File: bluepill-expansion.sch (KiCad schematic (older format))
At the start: 1 part, among them U1 BluePill_STM32F103C

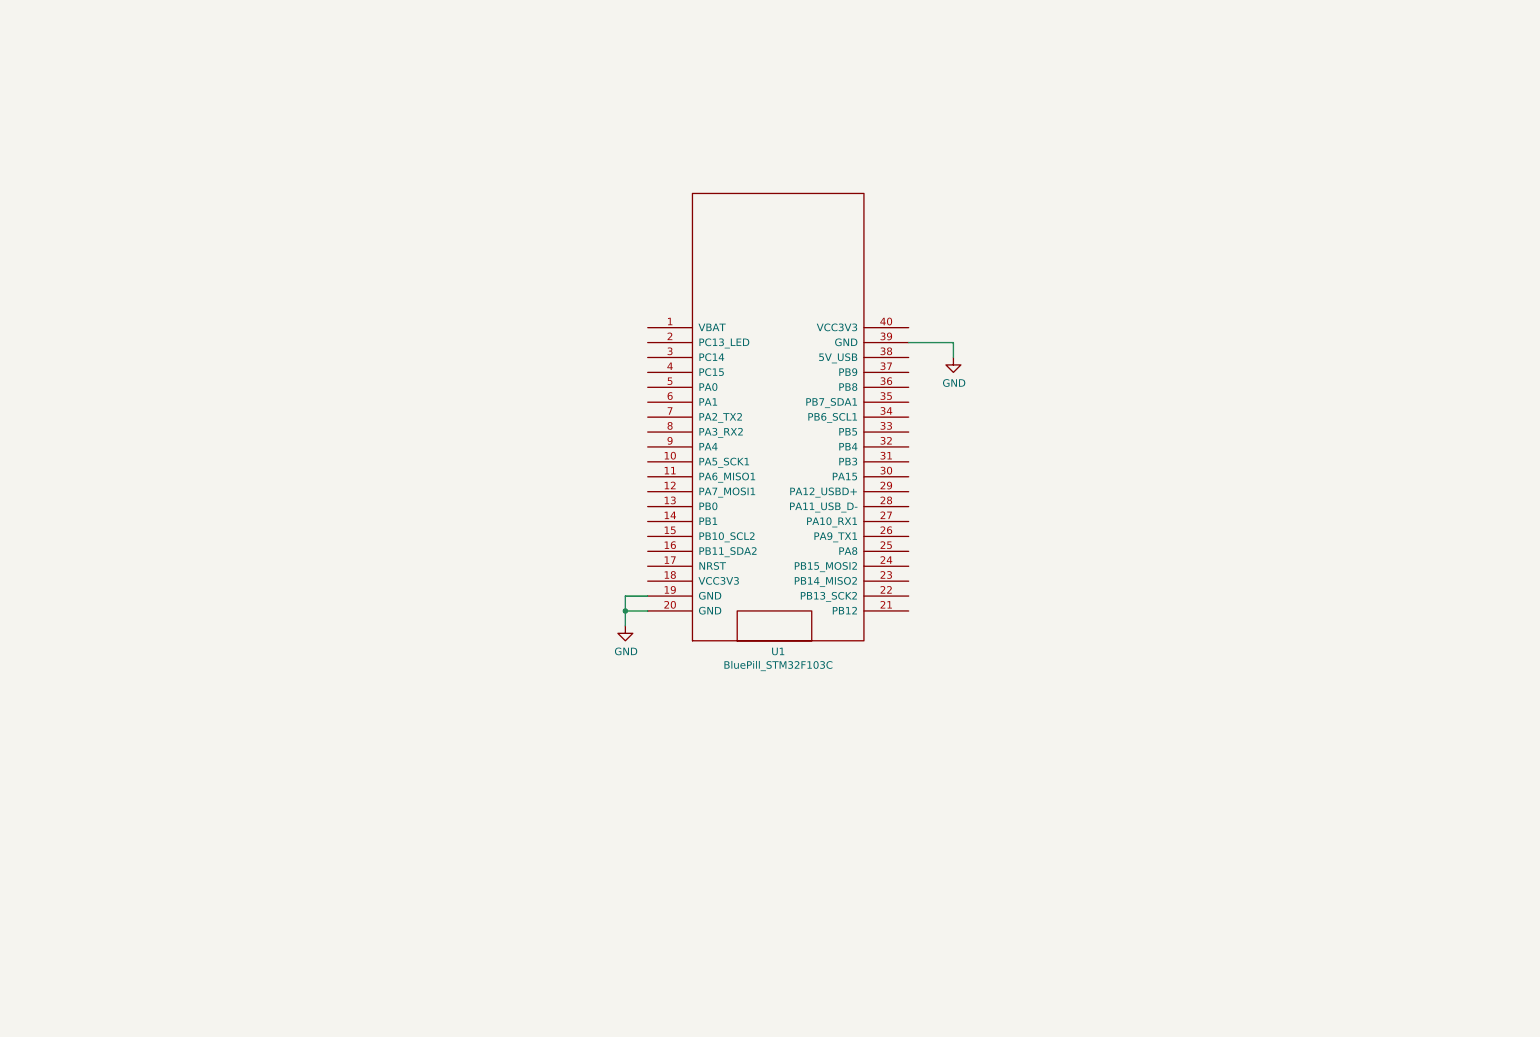
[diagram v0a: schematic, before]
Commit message: project update
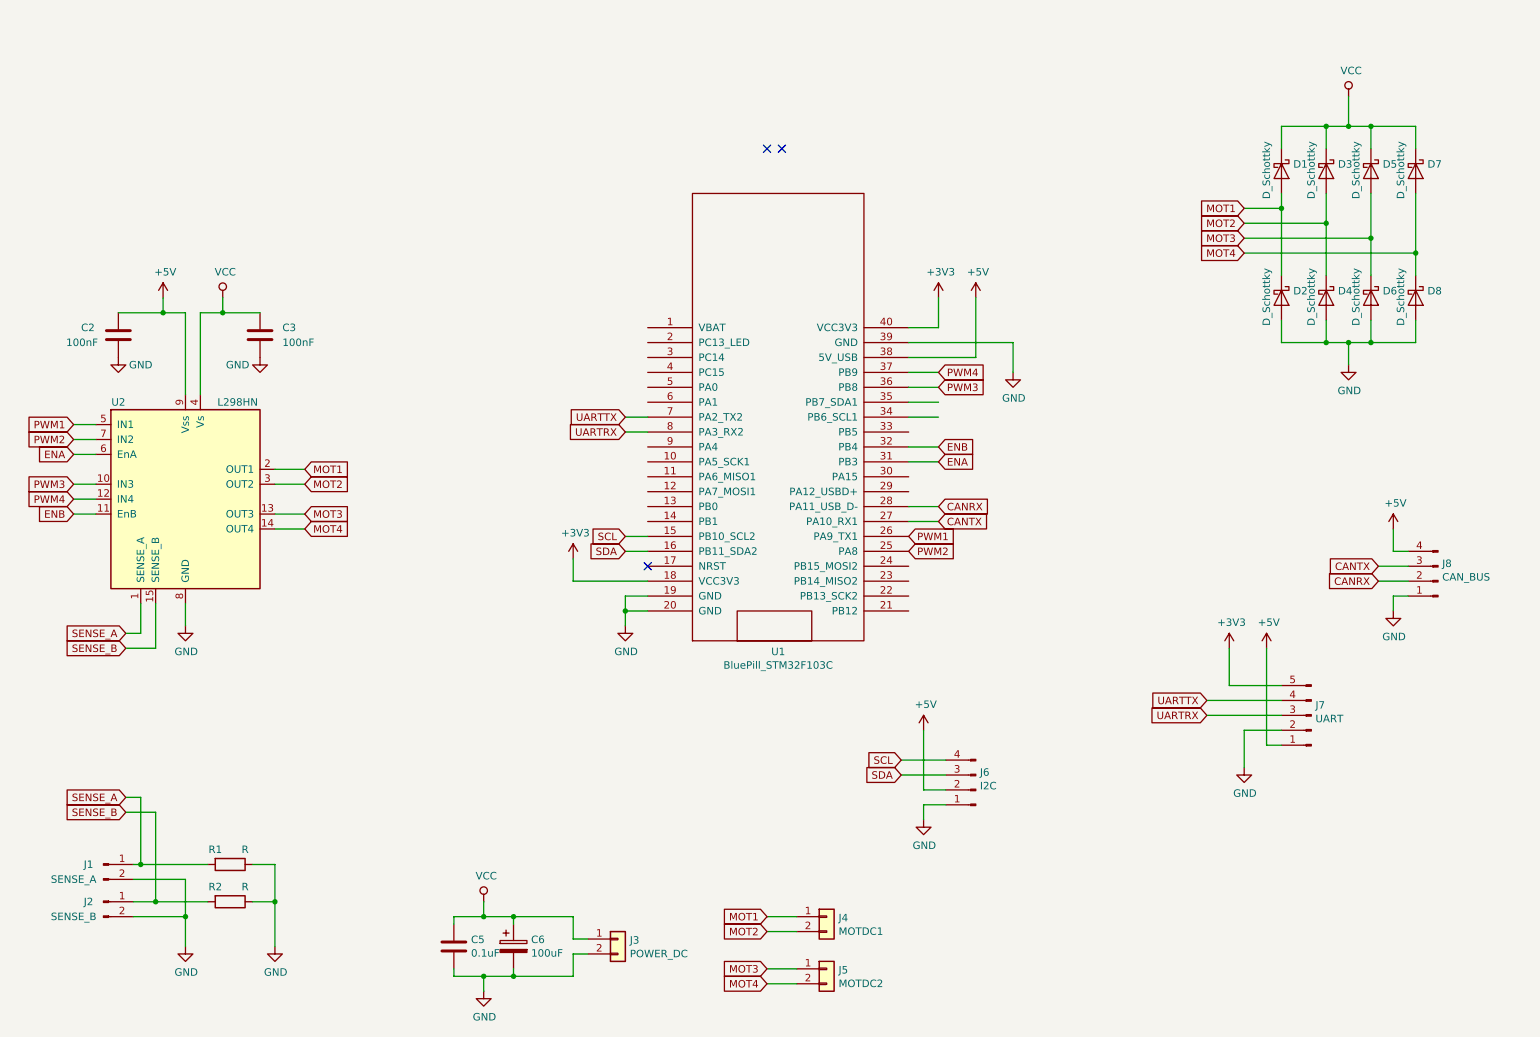
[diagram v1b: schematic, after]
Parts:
- added C2, C3: 100nF, symbol Device:C
- added C5: 0.1uF, Capacitor_THT:C_Disc_D7.5mm_W2.5mm_P5.00mm, symbol Device:C
- added C6: 100uF, Capacitor_THT:CP_Radial_D5.0mm_P2.50mm, symbol Device:CP
- added D1, D2, D3, D4, D5, D6, D7, D8: D_Schottky, symbol Device:D_Schottky
- added J1: SENSE_A, Connector_PinHeader_2.54mm:PinHeader_1x02_P2.54mm_Vertical, symbol Connector:Conn_01x02_Male
- added J2: SENSE_B, Connector_PinHeader_2.54mm:PinHeader_1x02_P2.54mm_Vertical, symbol Connector:Conn_01x02_Male
- added J3: POWER_DC, TerminalBlock:TerminalBlock_bornier-2_P5.08mm, symbol Connector_Generic:Conn_01x02
- added J4: MOTDC1, TerminalBlock:TerminalBlock_bornier-2_P5.08mm, symbol Connector_Generic:Conn_01x02
- added J5: MOTDC2, TerminalBlock:TerminalBlock_bornier-2_P5.08mm, symbol Connector_Generic:Conn_01x02
- added J6: I2C, Connector_PinHeader_2.54mm:PinHeader_1x04_P2.54mm_Vertical, symbol Connector:Conn_01x04_Male
- added J7: UART, Connector_PinHeader_2.54mm:PinHeader_1x05_P2.54mm_Vertical, symbol Connector:Conn_01x05_Male
- added J8: CAN_BUS, Connector_PinHeader_2.54mm:PinHeader_1x04_P2.54mm_Vertical, symbol Connector:Conn_01x04_Male
- added R1, R2: R, symbol Device:R
- added U2: L298HN, Package_TO_SOT_THT:TO-220-15_P2.54x2.54mm_StaggerOdd_Lead4.58mm_Vertical, symbol Driver_Motor:L298HN
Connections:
- net GND: now also C2.2, C3.2, C5.2, C6.2, D2.2 (A), D4.2 (A), D6.2 (A), D8.2 (A), J1.2 (Pin_2), J2.2 (Pin_2), J3.2 (Pin_2), J6.1 (Pin_1), J7.2 (Pin_2), J8.1 (Pin_1), R1.1, R2.1, U2.8 (GND)
- net SCL: now reaches U1.15 (PB10_SCL2)
- net SCL: now also J6.4 (Pin_4)
- net SDA: now reaches U1.16 (PB11_SDA2)
- net SDA: now also J6.3 (Pin_3)
- net +3V3: now reaches U1.18 (VCC3V3)
- net +3V3: now also U1.40 (VCC3V3), J7.5 (Pin_5)
- net PWM2: now reaches U1.25 (PA8)
- net PWM2: now also U2.7 (IN2)
- net PWM1: now reaches U1.26 (PA9_TX1)
- net PWM1: now also U2.5 (IN1)
- net CANTX: now reaches U1.27 (PA10_RX1)
- net CANTX: now also J8.3 (Pin_3)
- net CANRX: now reaches U1.28 (PA11_USB_D-)
- net CANRX: now also J8.2 (Pin_2)
- net ENA: now reaches U1.31 (PB3)
- net ENA: now also U2.6 (EnA)
- net ENB: now reaches U1.32 (PB4)
- net ENB: now also U2.11 (EnB)
- net PWM3: now reaches U1.36 (PB8)
- net PWM3: now also U2.10 (IN3)
- net PWM4: now reaches U1.37 (PB9)
- net PWM4: now also U2.12 (IN4)
- net +5V: now reaches U1.38 (5V_USB)
- net +5V: now also C2.1, J6.2 (Pin_2), J7.1 (Pin_1), J8.4 (Pin_4), U2.9 (Vss)
- net UARTTX: now reaches U1.7 (PA2_TX2)
- net UARTTX: now also J7.4 (Pin_4)
- net UARTRX: now reaches U1.8 (PA3_RX2)
- net UARTRX: now also J7.3 (Pin_3)
- new net MOT1: D1.2 (A), D2.1 (K), J4.1 (Pin_1), U2.2 (OUT1)
- new net MOT2: D3.2 (A), D4.1 (K), J4.2 (Pin_2), U2.3 (OUT2)
- new net MOT3: D5.2 (A), D6.1 (K), J5.1 (Pin_1), U2.13 (OUT3)
- new net MOT4: D7.2 (A), D8.1 (K), J5.2 (Pin_2), U2.14 (OUT4)
- new net SENSE_A: J1.1 (Pin_1), R1.2, U2.1 (SENSE_A)
- new net SENSE_B: J2.1 (Pin_1), R2.2, U2.15 (SENSE_B)
- new net VCC: C3.1, C5.1, C6.1, D1.1 (K), D3.1 (K), D5.1 (K), D7.1 (K), J3.1 (Pin_1), U2.4 (Vs)
- no-connect marks 0 -> 3

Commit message: updated schematic
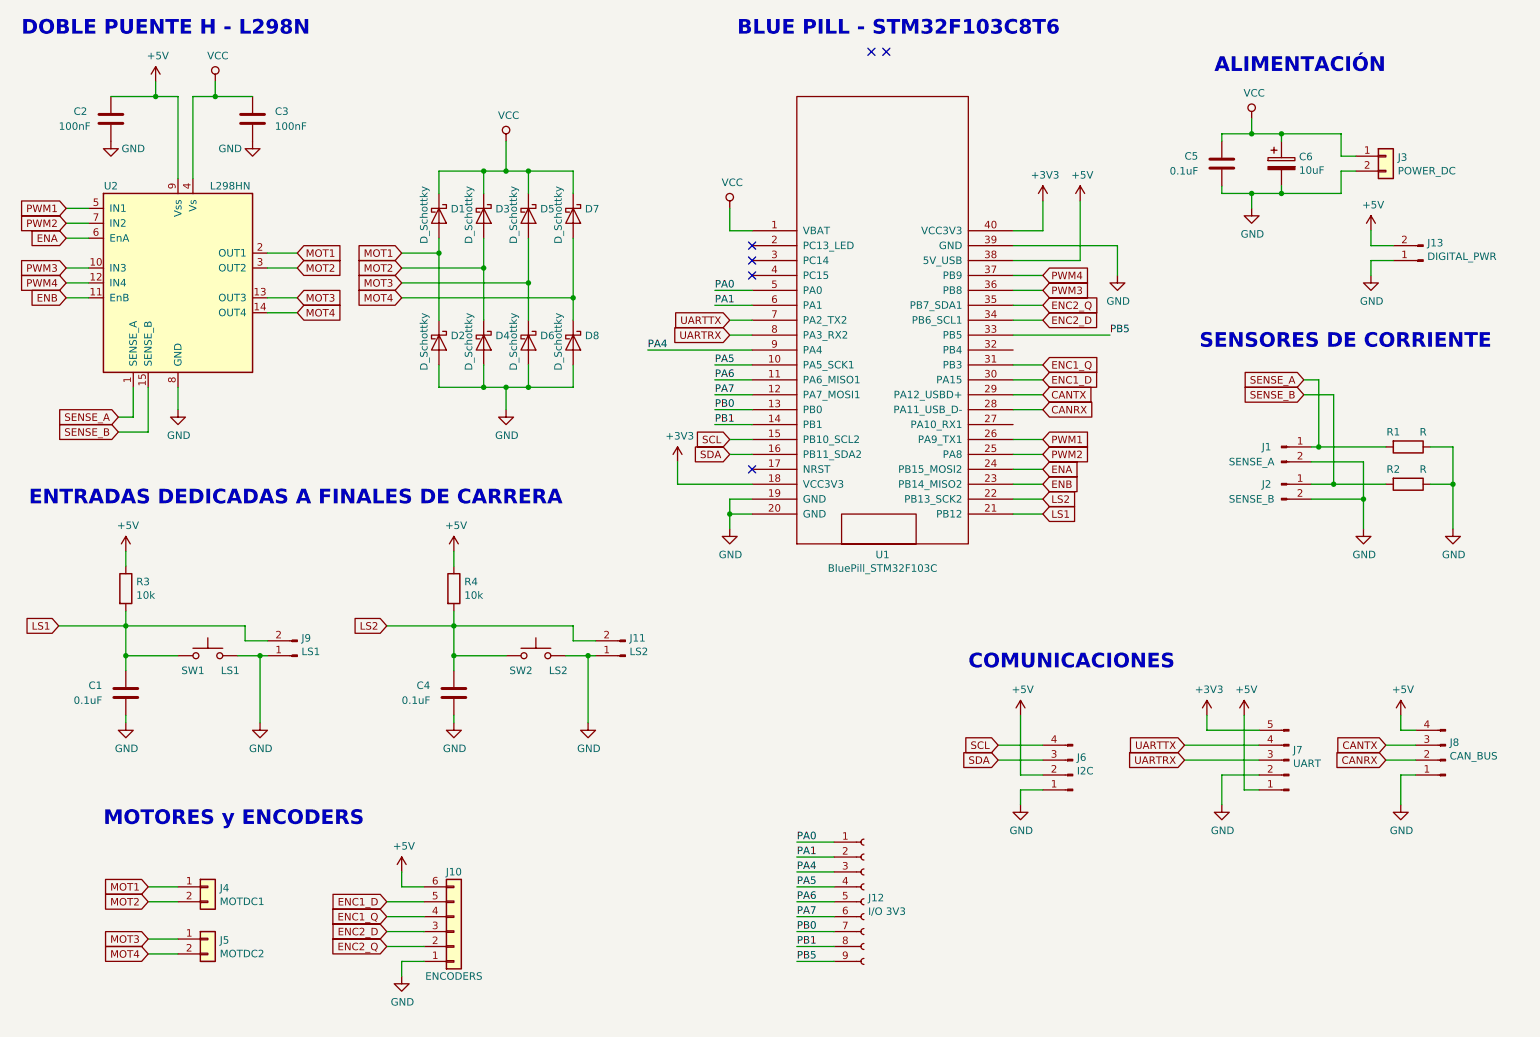
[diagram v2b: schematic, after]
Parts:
- added C1: 0.1uF, Capacitor_THT:C_Disc_D7.5mm_W2.5mm_P5.00mm, symbol Device:C
- added C4: 0.1uF, Capacitor_THT:C_Disc_D7.0mm_W2.5mm_P5.00mm, symbol Device:C
- added J10: ENCODERS, TerminalBlock:TerminalBlock_bornier-6_P5.08mm, symbol Connector_Generic:Conn_01x06
- added J11: LS2, Connector_PinHeader_2.54mm:PinHeader_1x02_P2.54mm_Vertical, symbol Connector:Conn_01x02_Male
- added J12: I/O 3V3, Connector_PinSocket_2.54mm:PinSocket_1x09_P2.54mm_Vertical, symbol Connector:Conn_01x09_Female
- added J13: DIGITAL_PWR, Connector_PinHeader_2.54mm:PinHeader_1x02_P2.54mm_Vertical, symbol Connector:Conn_01x02_Male
- added J9: LS1, Connector_PinHeader_2.54mm:PinHeader_1x02_P2.54mm_Vertical, symbol Connector:Conn_01x02_Male
- added R3, R4: 10k, Resistor_THT:R_Axial_DIN0207_L6.3mm_D2.5mm_P10.16mm_Horizontal, symbol Device:R
- added SW1: LS1, Button_Switch_THT:SW_PUSH_6mm_H8.5mm, symbol Switch:SW_Push
- added SW2: LS2, Button_Switch_THT:SW_PUSH_6mm_H8.5mm, symbol Switch:SW_Push
- C2, C3: footprint (none) -> Capacitor_THT:C_Disc_D7.5mm_W2.5mm_P5.00mm
- C6: value 100uF -> 10uF
- D1, D2, D3, D4, D5, D6, D7, D8: footprint (none) -> Diode_THT:D_DO-41_SOD81_P12.70mm_Horizontal
- R1, R2: footprint (none) -> Resistor_THT:R_Box_L26.0mm_W5.0mm_P20.00mm
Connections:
- net +5V: now also J10.6 (Pin_6), J13.2 (Pin_2), R3.1, R4.1
- net CANTX: now also U1.29 (PA12_USBD+); no longer U1.27 (PA10_RX1)
- net ENA: now also U1.24 (PB15_MOSI2); no longer U1.31 (PB3)
- net ENB: now also U1.23 (PB14_MISO2); no longer U1.32 (PB4)
- net GND: now also C1.2, C4.2, J10.1 (Pin_1), J11.1 (Pin_1), J13.1 (Pin_1), J9.1 (Pin_1), SW1.2, SW2.2
- net VCC: now also U1.1 (VBAT)
- net PA5: now reaches U1.10 (PA5_SCK1)
- net PA5: now also J12.4 (Pin_4)
- net PA6: now reaches U1.11 (PA6_MISO1)
- net PA6: now also J12.5 (Pin_5)
- net PA7: now reaches U1.12 (PA7_MOSI1)
- net PA7: now also J12.6 (Pin_6)
- net PB0: now reaches U1.13 (PB0)
- net PB0: now also J12.7 (Pin_7)
- net PB1: now reaches U1.14 (PB1)
- net PB1: now also J12.8 (Pin_8)
- net LS1: now reaches U1.21 (PB12)
- net LS1: now also C1.1, J9.2 (Pin_2), R3.2, SW1.1
- net LS2: now reaches U1.22 (PB13_SCK2)
- net LS2: now also C4.1, J11.2 (Pin_2), R4.2, SW2.1
- net ENC1_D: now reaches U1.30 (PA15)
- net ENC1_D: now also J10.5 (Pin_5)
- net PB5: now reaches U1.33 (PB5)
- net PB5: now also J12.9 (Pin_9)
- net ENC2_D: now reaches U1.34 (PB6_SCL1)
- net ENC2_D: now also J10.3 (Pin_3)
- net ENC2_Q: now reaches U1.35 (PB7_SDA1)
- net ENC2_Q: now also J10.2 (Pin_2)
- net PA0: now reaches U1.5 (PA0)
- net PA0: now also J12.1 (Pin_1)
- net PA1: now reaches U1.6 (PA1)
- net PA1: now also J12.2 (Pin_2)
- net PA4: now reaches U1.9 (PA4)
- net PA4: now also J12.3 (Pin_3)
- new net ENC1_Q: J10.4 (Pin_4), U1.31 (PB3)
- no-connect marks 3 -> 6
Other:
- note added: "ALIMENTACIÓN"
- note added: "BLUE PILL - STM32F103C8T6"
- note added: "COMUNICACIONES"
- note added: "DOBLE PUENTE H - L298N"
- note added: "ENTRADAS DEDICADAS A FINALES DE CARRERA"
- note added: "MOTORES y ENCODERS"
- note added: "SENSORES DE CORRIENTE"
- moved on the sheet: C2, C3, C5, C6, D1, D2, D3, D4, D5, D6, D7, D8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

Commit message: first routing
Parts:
- C4: footprint Capacitor_THT:C_Disc_D7.0mm_W2.5mm_P5.00mm -> Capacitor_THT:C_Disc_D7.5mm_W2.5mm_P5.00mm
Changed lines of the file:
@@
 F 0 "C4" H 3500 5450 50  0000 L CNN
 F 1 "0.1uF" H 3400 5350 50  0000 L CNN
-F 2 "Capacitor_THT:C_Disc_D7.0mm_W2.5mm_P5.00mm" H 3788 5250 50  0001 C CNN
+F 2 "Capacitor_THT:C_Disc_D7.5mm_W2.5mm_P5.00mm" H 3788 5250 50  0001 C CNN
 F 3 "~" H 3750 5400 50  0001 C CNN
 	1    3750 5400

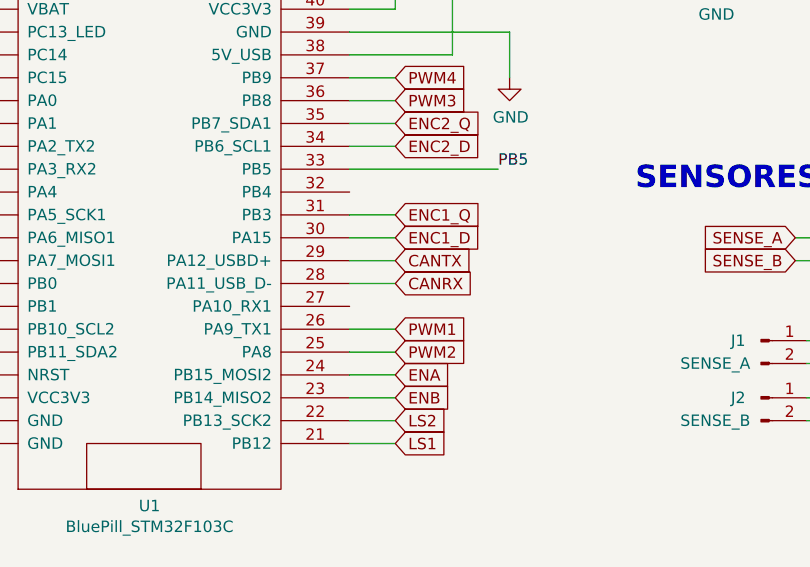
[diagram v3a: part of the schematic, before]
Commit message: final routing sin revisar
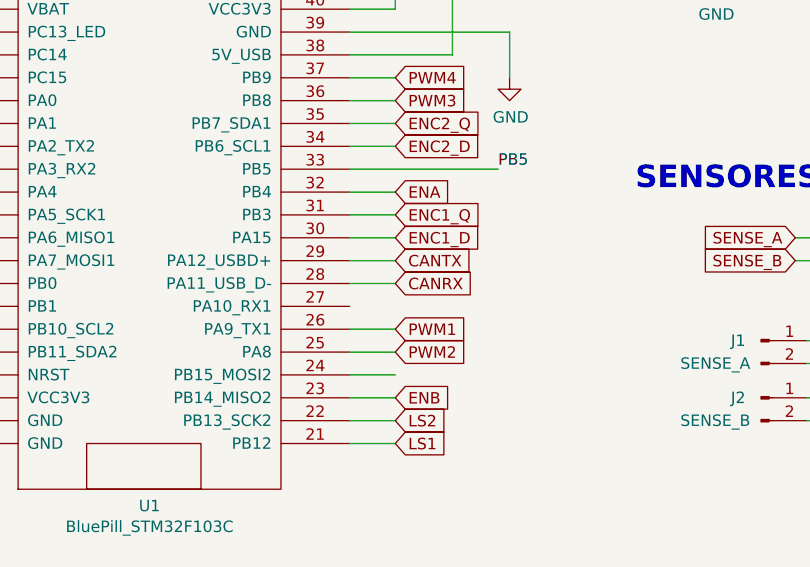
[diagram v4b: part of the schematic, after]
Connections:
- net ENA: now also U1.32 (PB4); no longer U1.24 (PB15_MOSI2)
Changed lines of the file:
@@
 Wire Wire Line
 	7500 2600 7700 2600
-Text GLabel 7700 3900 2    50   Input ~ 0
+Text GLabel 7700 3100 2    50   Input ~ 0
 ENA
 Wire Wire Line
@@
 Text Notes 1400 6300 0    98   ~ 20
 MOTORES y ENCODERS
+Wire Wire Line
+	7500 3100 7700 3100
 $EndSCHEMATC
